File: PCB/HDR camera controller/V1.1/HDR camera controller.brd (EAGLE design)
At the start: 58 x 48 mm, 63 parts, among them IC1 USBLC6-4, IC10 RS422-SO8, IC11 RS422-SO8, IC12 USBLC6-4, IC14 741G157, IC2 RS422-SO8, IC3 RS422-SO8, IC4 RS422-SO8, IC6 FT232RL, IC7 74HC00D, IC8 74HC139D, IC9 RS422-SO8, Q1 16MHz

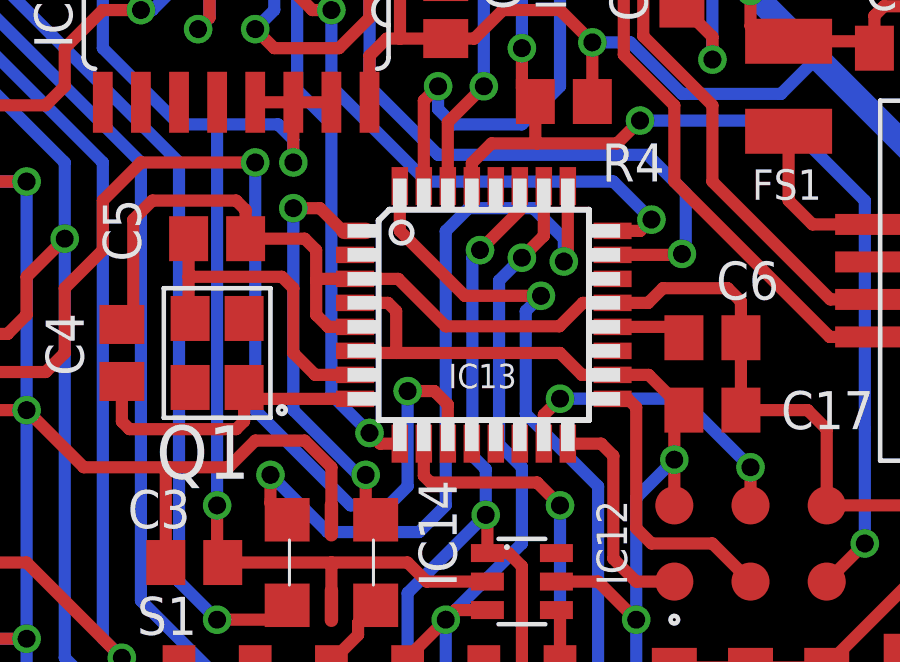
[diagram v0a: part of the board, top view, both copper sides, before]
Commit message: wip
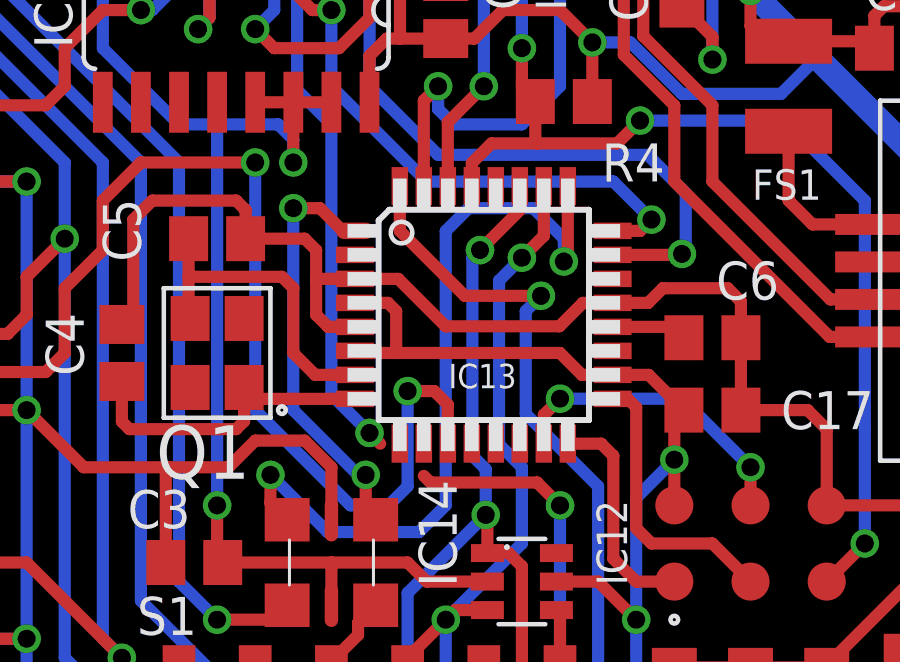
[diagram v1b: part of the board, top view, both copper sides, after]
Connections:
- net ENC_B: now also IC13.2; no longer IC13.27
- net LINE_IN_1: now also IC13.13; no longer IC13.10
- net L_IN: now also IC13.14; no longer IC13.9
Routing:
- net LINE_IN_1: track 35.5 -> 34.4 mm
- net ENC_B: track 94.1 -> 93.3 mm
- net L_IN: track 33.1 -> 32.5 mm
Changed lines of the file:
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@@
 </layers>
 <board>
-<fusionsync huburn="a.cGVyc29uYWw6dWUyYWFhMjdi" projecturn="a.cGVyc29uYWw6dWUyYWFhMjdiIzIwMTcxMTIzMTA1NDAxMzMx" f3durn="urn:adsk.wipprod:dm.lineage:Xuph5AAnRz6wK6HHSwnN2A" pcbguid="" lastpulledtime="" lastsyncedchangeguid="" latestrevisionid="6616cd26-1267-4b75-a275-6117032d61cd" lastsyncedrevisionid="6616cd26-1267-4b75-a275-6117032d61cd" lastboardhashguid="059826bd-0402-169d-34a1-e7c392c3920d" lastpushedtime="2021-12-01T15:11:12Z" linktopcb3d="true"/>
+<fusionsync huburn="a.cGVyc29uYWw6dWUyYWFhMjdi" projecturn="a.cGVyc29uYWw6dWUyYWFhMjdiIzIwMTcxMTIzMTA1NDAxMzMx" f3durn="urn:adsk.wipprod:dm.lineage:Xuph5AAnRz6wK6HHSwnN2A" pcbguid="" lastpulledtime="" lastsyncedchangeguid="" latestrevisionid="6616cd26-1267-4b75-a275-6117032d61cd" lastsyncedrevisionid="6616cd26-1267-4b75-a275-6117032d61cd" lastboardhashguid="059826bd-0402-169d-34a1-e7c392c3920d" lastpushedtime="2021-12-01T15:11:12Z" linktopcb3d="false"/>
 <plain>
 <wire x1="0" y1="44.5" x2="0" y2="3.5" width="0" layer="20"/>
@@
 <contactref element="IC2" pad="3"/>
 <contactref element="R2" pad="2"/>
-<contactref element="IC13" pad="10"/>
 <wire x1="17.0434" y1="6.985" x2="20.32" y2="6.985" width="0.4064" layer="1"/>
 <wire x1="20.32" y1="6.985" x2="20.955" y2="6.985" width="0.4064" layer="1"/>
@@
 <wire x1="24.13" y1="6.35" x2="21.59" y2="6.35" width="0.4064" layer="1"/>
 <wire x1="21.59" y1="6.35" x2="20.955" y2="6.985" width="0.4064" layer="1"/>
-<wire x1="32.29" y1="18.5674" x2="32.29" y2="17.494" width="0.4064" layer="1"/>
 <wire x1="36.83" y1="16.51" x2="36.068" y2="17.272" width="0.4064" layer="1"/>
 <wire x1="36.068" y1="17.272" x2="32.512" y2="17.272" width="0.4064" layer="1"/>
@@
 <wire x1="32.29" y1="17.494" x2="32.512" y2="17.272" width="0.4064" layer="1"/>
 <wire x1="36.83" y1="8.89" x2="33.909" y2="5.969" width="0.4064" layer="16"/>
+<contactref element="IC13" pad="13"/>
+<wire x1="32.29" y1="17.494" x2="34.69" y2="18.5674" width="0" layer="19" extent="1-1"/>
 </signal>
 <signal name="LINE_OUT_1">
@@
 <contactref element="IC7" pad="12"/>
 <contactref element="R7" pad="2"/>
-<contactref element="IC13" pad="9"/>
 <wire x1="26.67" y1="38.8366" x2="27.94" y2="38.8366" width="0.4064" layer="1"/>
 <wire x1="27.94" y1="40.259" x2="27.94" y2="38.8366" width="0.4064" layer="1"/>
@@
 <wire x1="29.21" y1="41.529" x2="29.21" y2="36.83" width="0.4064" layer="16"/>
 <wire x1="29.21" y1="36.83" x2="28.067" y2="35.687" width="0.4064" layer="16"/>
-<wire x1="31.49" y1="18.5674" x2="30.8356" y2="18.5674" width="0.4064" layer="1"/>
 <wire x1="30.8356" y1="18.5674" x2="30.48" y2="18.923" width="0.4064" layer="1"/>
 <via x="30.48" y="18.923" extent="1-16" drill="0.6"/>
 <wire x1="30.48" y1="18.923" x2="29.21" y2="20.193" width="0.4064" layer="16"/>
 <wire x1="29.21" y1="20.193" x2="29.21" y2="29.21" width="0.4064" layer="16"/>
+<contactref element="IC13" pad="14"/>
+<wire x1="30.8356" y1="18.5674" x2="35.49" y2="18.5674" width="0" layer="19" extent="1-1"/>
 </signal>
 <signal name="L_SEL0">
@@
 <contactref element="TRIG" pad="3"/>
 <contactref element="IC4" pad="3"/>
-<contactref element="IC13" pad="27"/>
 <wire x1="2.54" y1="34.29" x2="8.89" y2="34.29" width="0.4064" layer="1"/>
 <via x="8.89" y="34.29" extent="1-16" drill="0.6"/>
@@
 <wire x1="35.56" y1="11.176" x2="35.2298" y2="10.8458" width="0.4064" layer="1"/>
 <wire x1="35.2298" y1="10.8458" x2="34.29" y2="10.8458" width="0.4064" layer="1"/>
-<wire x1="35.49" y1="27.1526" x2="35.49" y2="26.346" width="0.4064" layer="1"/>
 <via x="34.163" y="25.019" extent="1-16" drill="0.6"/>
 <wire x1="34.163" y1="25.019" x2="33.909" y2="24.765" width="0.4064" layer="16"/>
-<wire x1="35.49" y1="26.346" x2="34.163" y2="25.019" width="0.4064" layer="1"/>
+<wire x1="35.49" y1="26.346" x2="34.417" y2="25.273" width="0.4064" layer="1"/>
+<wire x1="34.417" y1="25.273" x2="34.163" y2="25.019" width="0.4064" layer="1"/>
 <wire x1="33.909" y1="24.765" x2="33.909" y2="18.161" width="0.4064" layer="16"/>
 <wire x1="34.3535" y1="17.7165" x2="33.909" y2="18.161" width="0.4064" layer="16"/>
@@
 <via x="22.225" y="11.43" extent="1-16" drill="0.6"/>
 <wire x1="19.05" y1="14.605" x2="22.225" y2="11.43" width="0.4064" layer="1"/>
+<contactref element="IC13" pad="2"/>
+<wire x1="34.417" y1="25.273" x2="29.9974" y2="24.86" width="0" layer="19" extent="1-1"/>
 </signal>
 <signal name="ENC_A">
